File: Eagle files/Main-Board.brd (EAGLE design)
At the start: 76.2 x 81.3 mm, 58 parts, among them J3 POWER_JACKPTH, J4 AVR_SPI_PRG_62X3_LOCK, Q1 DMN3404L, Q2 DMN3404L, Q3 DMN3404L, Q4 MMBT2222A, U1 ATMEGA328P, Y1 16mhz

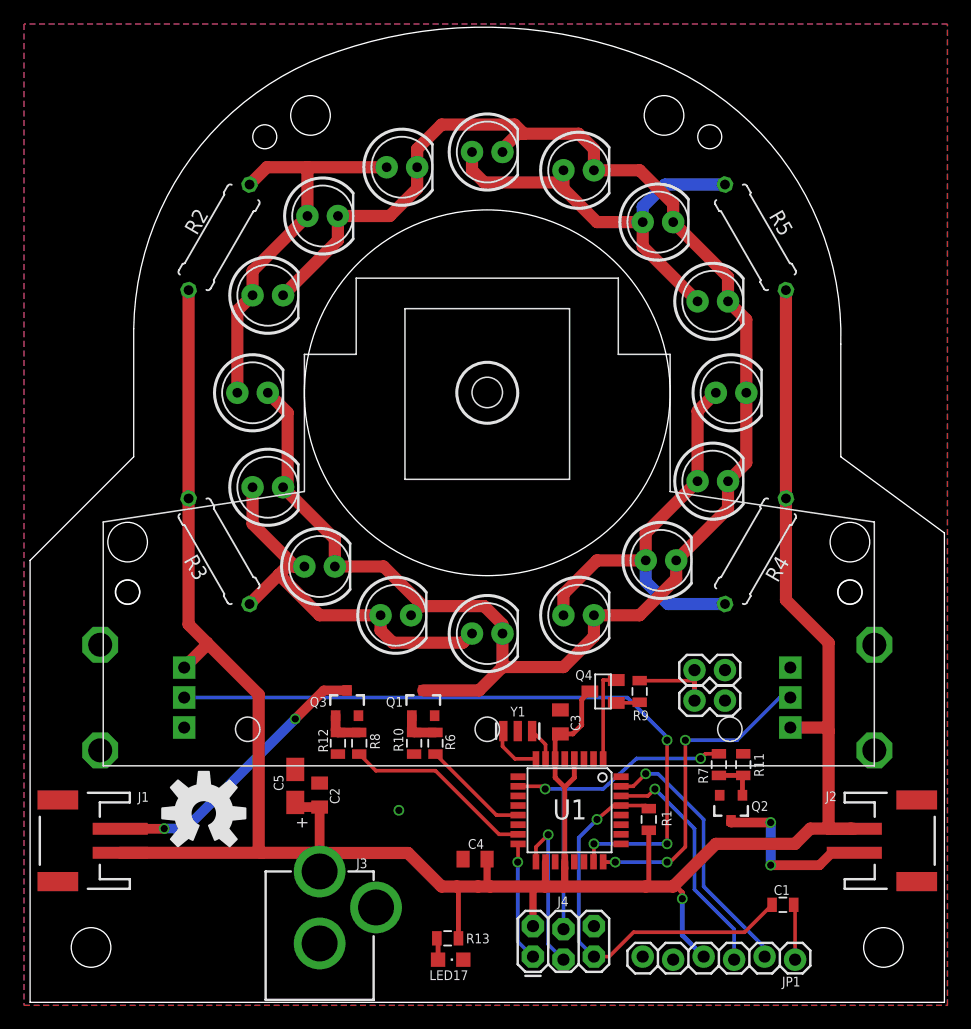
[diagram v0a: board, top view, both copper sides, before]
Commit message: Updated Eagle files + BOMs
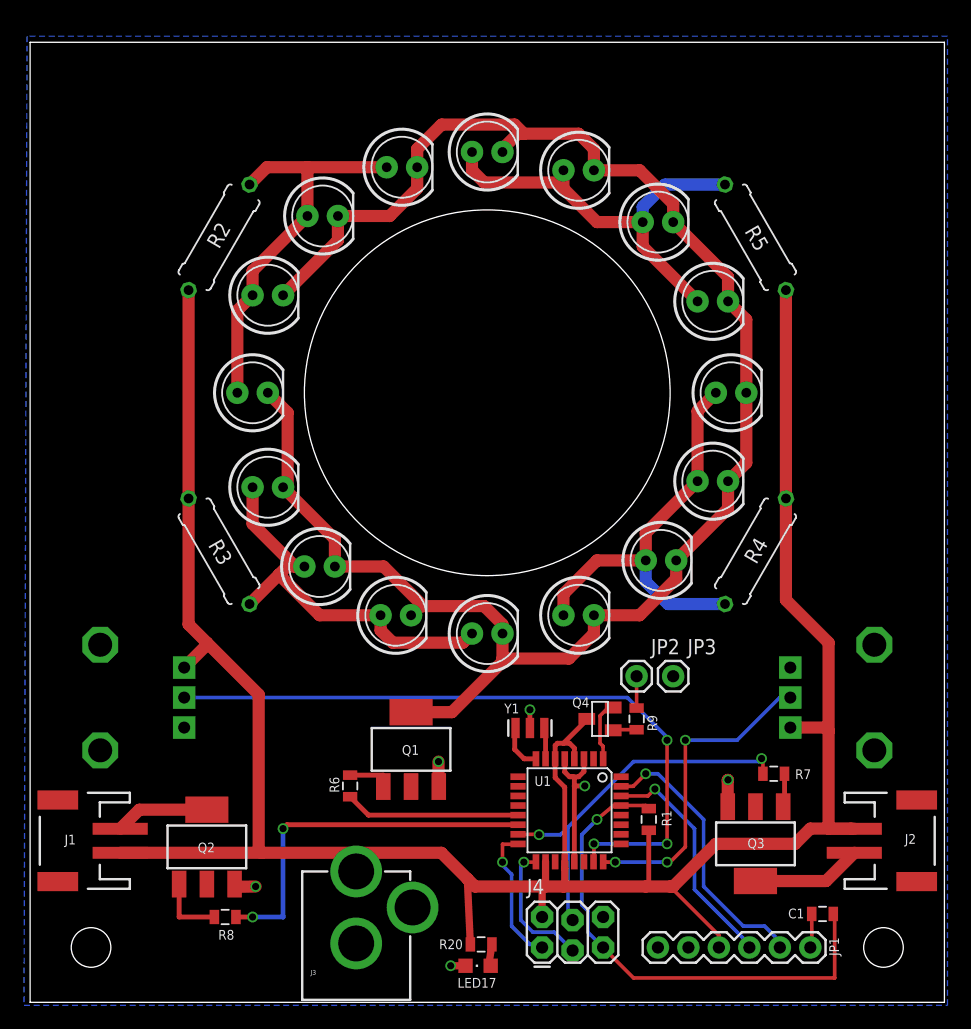
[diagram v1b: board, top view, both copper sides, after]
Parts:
- removed C2, C3, C4: 0.1uF, adafruit:C0805K
- removed C5: 10uF, adafruit:A/3216-18R
- removed JP4: (no value), SparkFun-Connectors:1X02
- removed LOGO1: OSHW-LOGOL, SparkFun-Aesthetics:OSHW-LOGO-L
- removed R10: 10k, SparkFun-Resistors:0805
- removed R13: 82, SparkFun-Resistors:0805
- removed R14, R15: 10k, SparkFun-Electromechanical:ALPS_POT
- removed STANDOFF3, STANDOFF4, STANDOFF5, STANDOFF6: STAND-OFF, SparkFun-Electromechanical:STAND-OFF
- removed U$1: PS3EYE, ps3eye:PS3EYE
- added JP3: GND, SparkFun-Connectors:1X01
- added R20: 10k, SparkFun-Resistors:0805
- added U$4: PS3EYE, ps3eye:PS3EYE
- JP1: value (none) -> FTDI_BASICPTH; device SparkFun-Connectors:1X06_LOCK -> SparkFun-Connectors:FTDI_BASIC
- JP2: value (none) -> VSYNC; device SparkFun-Connectors:1X02 -> SparkFun-Connectors:1X01
- Q1, Q2, Q3: device SparkFun-DiscreteSemi:SOT23-3 -> transistor-power:SOT223
- R11, R12: device SparkFun-Resistors:0805 -> SparkFun-Electromechanical:ALPS_POT
- R6, R7, R8: value 220ohm -> 100ohm
- moved Q2 43.8 mm to (14.7, 13.0), turned to 0 degrees
- moved Q3 36.0 mm to (60.5, 13.2), turned to 180 degrees
- moved R12 20.2 mm to (5.84, 25.4), turned to 0 degrees
- moved R8 18.3 mm to (16.3, 7.11), turned to 180 degrees
- moved R11 12.3 mm to (70.4, 25.4), turned to 180 degrees
- moved R6 7.95 mm to (26.7, 18.0)
- moved JP2 4.85 mm to (50.5, 27.2)
- moved R7 4.64 mm to (62.0, 19.1), turned to 0 degrees
- moved Q1 3.94 mm to (31.8, 21.1)
- moved C1 3.39 mm to (66.0, 7.37), turned to 180 degrees
- moved J3 3.05 mm to (27.2, -2.79)
- moved LED17 2.34 mm to (37.3, 3.05), turned to 90 degrees
- moved Q4 2.30 mm to (47.5, 23.6)
- moved R9 2.30 mm to (50.5, 23.6)
- moved JP1 1.63 mm to (65.0, 4.57)
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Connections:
- removed net N$12: JP2.1, JP4.1, R9.2
- new net N$17: JP2.1, R9.2
- net 5V: now also JP1.VCC, R11.P$3, R12.P$3, R20.2; no longer C2.1, C3.1, C4.1, C5.+, JP1.4, R13.2, R14.P$3, R15.P$3
- net GLINT_RIGHT: now also U1.14; no longer U1.15
- net GND: now also JP1.CTS, JP1.GND, JP3.1, Q1.3, Q2.3, Q3.3, R11.P$1, R12.P$1; no longer C2.2, C3.2, C4.2, C5.-, JP1.5, JP1.6, JP2.2, JP4.2, Q1.2, Q2.2, Q3.2, R10.2, R11.2, R12.2, R14.P$1, R15.P$1
- net LEFT_BRIGHTNESS: now also R12.P$2; no longer R14.P$2
- net MOSI: now also U1.15; no longer U1.10
- net N$1: now also R20.1; no longer R13.1
- net N$11: now also Q2.4; no longer Q3.3
- net N$13: now also Q1.4; no longer Q1.3
- net N$14: now also Q2.1; no longer Q3.1, R12.1
- net N$16: now also JP1.DTR; no longer JP1.1
- net N$5: now also Q3.4; no longer Q2.3
- net N$7: no longer R10.1
- net N$9: now also Q3.1; no longer Q2.1, R11.1
- net RIGHT_BRIGHTNESS: now also R11.P$2; no longer R15.P$2
- net RXI: now also JP1.RXI; no longer JP1.2
- net TXO: now also JP1.TXO; no longer JP1.3
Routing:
- net GND: track 0.00 -> 21.1 mm, vias 1 -> 6
- net N$11: track 23.7 -> 7.88 mm, vias 2 -> 0
- net GLINT_RIGHT: track 16.0 -> 31.0 mm, vias 0 -> 2
- net 5V: track 220.6 -> 207.8 mm, vias 1 -> 0
- net RESET: track 34.1 -> 42.6 mm
- net N$12: track 7.25 -> 0.00 mm
- net LED_RING: track 8.99 -> 14.6 mm
- net N$5: track 14.5 -> 9.21 mm, vias 2 -> 0
- net N$17: track 0.00 -> 2.66 mm
- net VSYNC_IN: track 7.66 -> 5.08 mm
- net MOSI: track 29.7 -> 32.2 mm
- net N$14: track 3.26 -> 5.68 mm
- net SCK: track 13.6 -> 11.3 mm
- net MISO: track 9.93 -> 11.7 mm
- net N$16: track 4.69 -> 3.13 mm
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- removed copper zone on layer 1, net GND
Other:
- board size 76.2 x 81.3 mm -> 76.2 x 80 mm
- board text added: "BRIGHTNESS"
- board text added: "LEFT"
- board text removed: "(REV A)"
- board text removed: "<FTDI 5V>"
- board text removed: "BLK"
- board text removed: "Designed by"
- board text removed: "EYEWRITER 2.1"
- board text removed: "Eyewriter 2.1"
- board text removed: "GND"
- board text removed: "GRN"
- board text removed: "Jason Webb"
- board text removed: "MAIN BOARD"
- board text removed: "MISO"
- board text removed: "Main board"
- board text removed: "OSHW"
- board text removed: "RST"
- board text removed: "SCK"
- board text removed: "VSYNC"
- board text removed: "http://jason-webb.info"

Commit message: Updated Eagle files, including Gerbers and custom library
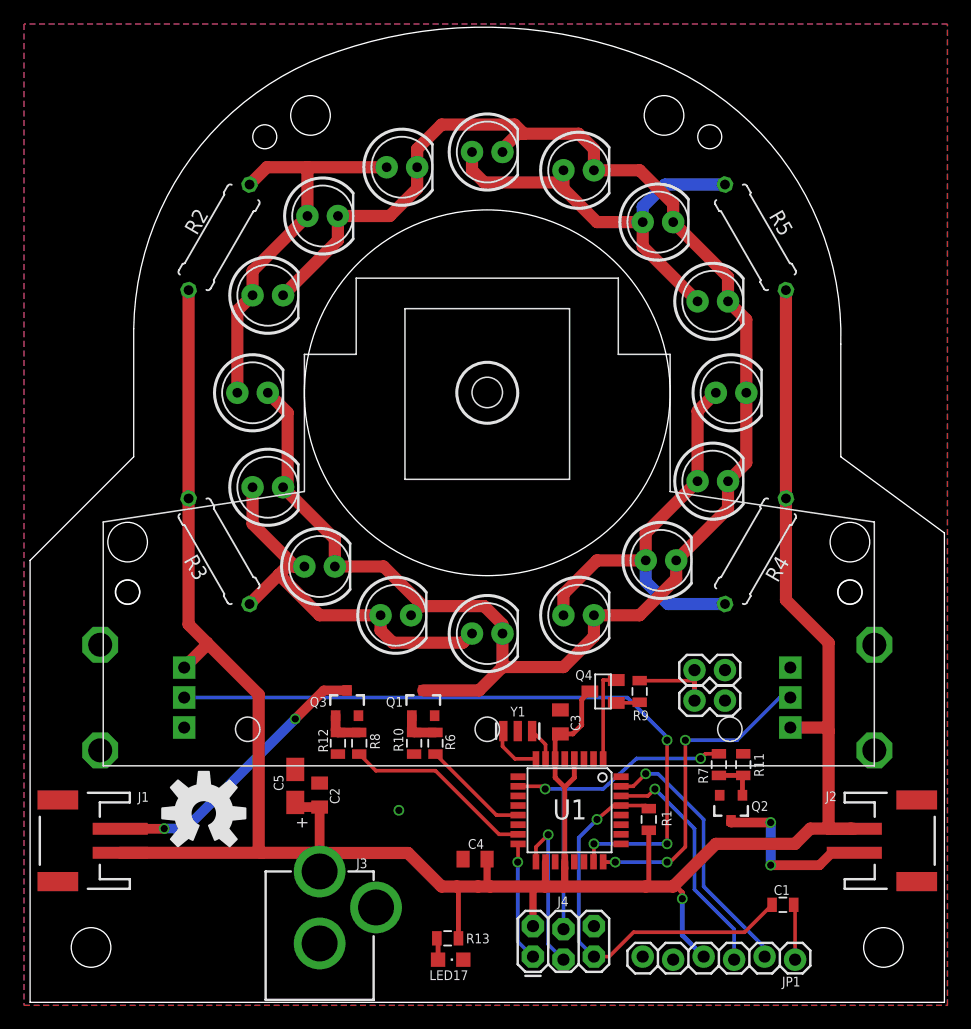
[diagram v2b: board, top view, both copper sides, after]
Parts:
- removed JP3: GND, SparkFun-Connectors:1X01
- removed R20: 10k, SparkFun-Resistors:0805
- removed U$4: PS3EYE, ps3eye:PS3EYE
- added C2, C3, C4: 0.1uF, adafruit:C0805K
- added C5: 10uF, adafruit:A/3216-18R
- added JP4: (no value), SparkFun-Connectors:1X02
- added LOGO1: OSHW-LOGOL, SparkFun-Aesthetics:OSHW-LOGO-L
- added R10: 10k, SparkFun-Resistors:0805
- added R13: 82, SparkFun-Resistors:0805
- added R14, R15: 10k, SparkFun-Electromechanical:ALPS_POT
- added STANDOFF3, STANDOFF4, STANDOFF5, STANDOFF6: STAND-OFF, SparkFun-Electromechanical:STAND-OFF
- added U$1: PS3EYE, ps3eye:PS3EYE
- JP1: value FTDI_BASICPTH -> (none); device SparkFun-Connectors:FTDI_BASIC -> SparkFun-Connectors:1X06_LOCK
- JP2: value VSYNC -> (none); device SparkFun-Connectors:1X01 -> SparkFun-Connectors:1X02
- Q1, Q2, Q3: device transistor-power:SOT223 -> SparkFun-DiscreteSemi:SOT23-3
- R11, R12: device SparkFun-Electromechanical:ALPS_POT -> SparkFun-Resistors:0805
- R6, R7, R8: value 100ohm -> 220ohm
- moved Q2 43.8 mm to (58.4, 16.3), turned to 180 degrees
- moved Q3 36.0 mm to (26.4, 24.9), turned to 0 degrees
- moved R12 20.2 mm to (25.7, 21.6), turned to 270 degrees
- moved R8 18.3 mm to (27.4, 21.6), turned to 90 degrees
- moved R11 12.3 mm to (59.4, 19.8), turned to 90 degrees
- moved R6 7.95 mm to (33.8, 21.6)
- moved JP2 4.85 mm to (55.4, 27.7)
- moved R7 4.64 mm to (57.4, 19.8), turned to 270 degrees
- moved Q1 3.94 mm to (32.8, 24.9)
- moved C1 3.39 mm to (62.7, 8.13), turned to 0 degrees
- moved J3 3.05 mm to (24.1, -2.79)
- moved LED17 2.34 mm to (35.1, 3.56), turned to 270 degrees
- moved Q4 2.30 mm to (47.8, 25.9)
- moved R9 2.30 mm to (50.8, 25.9)
- moved JP1 1.63 mm to (63.8, 3.56)
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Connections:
- removed net N$17: JP2.1, R9.2
- new net N$12: JP2.1, JP4.1, R9.2
- net 5V: now also C2.1, C3.1, C4.1, C5.+, JP1.4, R13.2, R14.P$3, R15.P$3; no longer JP1.VCC, R11.P$3, R12.P$3, R20.2
- net GLINT_RIGHT: now also U1.15; no longer U1.14
- net GND: now also C2.2, C3.2, C4.2, C5.-, JP1.5, JP1.6, JP2.2, JP4.2, Q1.2, Q2.2, Q3.2, R10.2, R11.2, R12.2, R14.P$1, R15.P$1; no longer JP1.CTS, JP1.GND, JP3.1, Q1.3, Q2.3, Q3.3, R11.P$1, R12.P$1
- net LEFT_BRIGHTNESS: now also R14.P$2; no longer R12.P$2
- net MOSI: now also U1.10; no longer U1.15
- net N$1: now also R13.1; no longer R20.1
- net N$11: now also Q3.3; no longer Q2.4
- net N$13: now also Q1.3; no longer Q1.4
- net N$14: now also Q3.1, R12.1; no longer Q2.1
- net N$16: now also JP1.1; no longer JP1.DTR
- net N$5: now also Q2.3; no longer Q3.4
- net N$7: now also R10.1
- net N$9: now also Q2.1, R11.1; no longer Q3.1
- net RIGHT_BRIGHTNESS: now also R15.P$2; no longer R11.P$2
- net RXI: now also JP1.2; no longer JP1.RXI
- net TXO: now also JP1.3; no longer JP1.TXO
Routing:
- net GND: track 21.1 -> 0.00 mm, vias 6 -> 1
- net N$11: track 7.88 -> 23.7 mm, vias 0 -> 2
- net GLINT_RIGHT: track 31.0 -> 16.0 mm, vias 2 -> 0
- net 5V: track 207.8 -> 220.6 mm, vias 0 -> 1
- net RESET: track 42.6 -> 34.1 mm
- net N$12: track 0.00 -> 7.25 mm
- net LED_RING: track 14.6 -> 8.99 mm
- net N$5: track 9.21 -> 14.5 mm, vias 0 -> 2
- net N$17: track 2.66 -> 0.00 mm
- net VSYNC_IN: track 5.08 -> 7.66 mm
- net MOSI: track 32.2 -> 29.7 mm
- net N$14: track 5.68 -> 3.26 mm
- net SCK: track 11.3 -> 13.6 mm
- net MISO: track 11.7 -> 9.93 mm
- net N$16: track 3.13 -> 4.69 mm
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- added copper zone on layer 1, net GND
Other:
- board size 76.2 x 80 mm -> 76.2 x 81.3 mm
- board text added: "(REV A)"
- board text added: "<FTDI 5V>"
- board text added: "BLK"
- board text added: "Designed by"
- board text added: "EYEWRITER 2.1"
- board text added: "Eyewriter 2.1"
- board text added: "GND"
- board text added: "GRN"
- board text added: "Jason Webb"
- board text added: "MAIN BOARD"
- board text added: "MISO"
- board text added: "Main board"
- board text added: "OSHW"
- board text added: "RST"
- board text added: "SCK"
- board text added: "VSYNC"
- board text added: "http://jason-webb.info"
- board text removed: "BRIGHTNESS"
- board text removed: "LEFT"
